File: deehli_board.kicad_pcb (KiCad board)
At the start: 2 copper layers, 84 x 51 mm, 46 parts, among them J1 Servo_Out, J2 PWM_In, J3 Vcc_Out, J4 Conn_01x08_Socket, J5 CAN_Ext, J6 Board_IO, J7 Conn_01x08_Socket, SW1 SW_DPDT_x2, U1 APE1707M-50-HF, U2 LM2576HVT-5, U3 LM2576HVT-5, U4 LM2576HVT-15, U5 LD1117S33TR_SOT223, U6 LM2576HVT-15

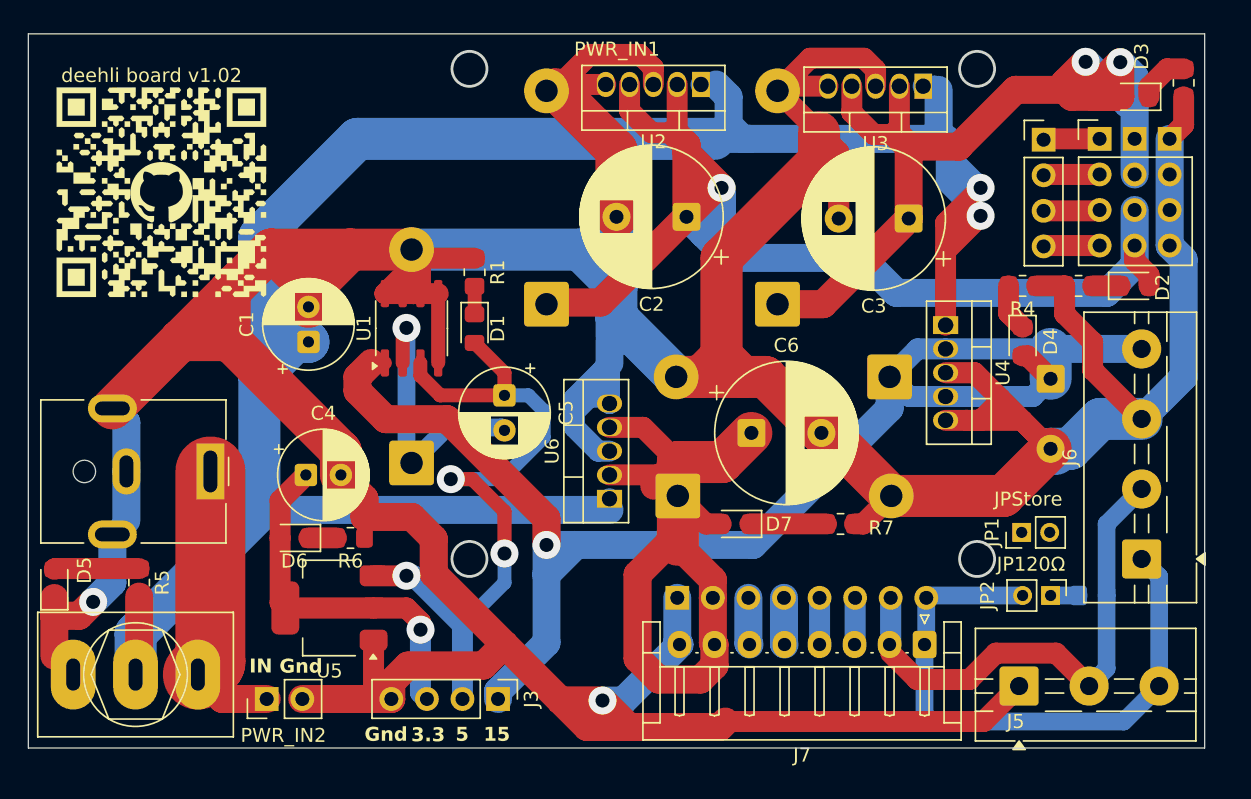
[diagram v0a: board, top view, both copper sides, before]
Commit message: vB-1.01
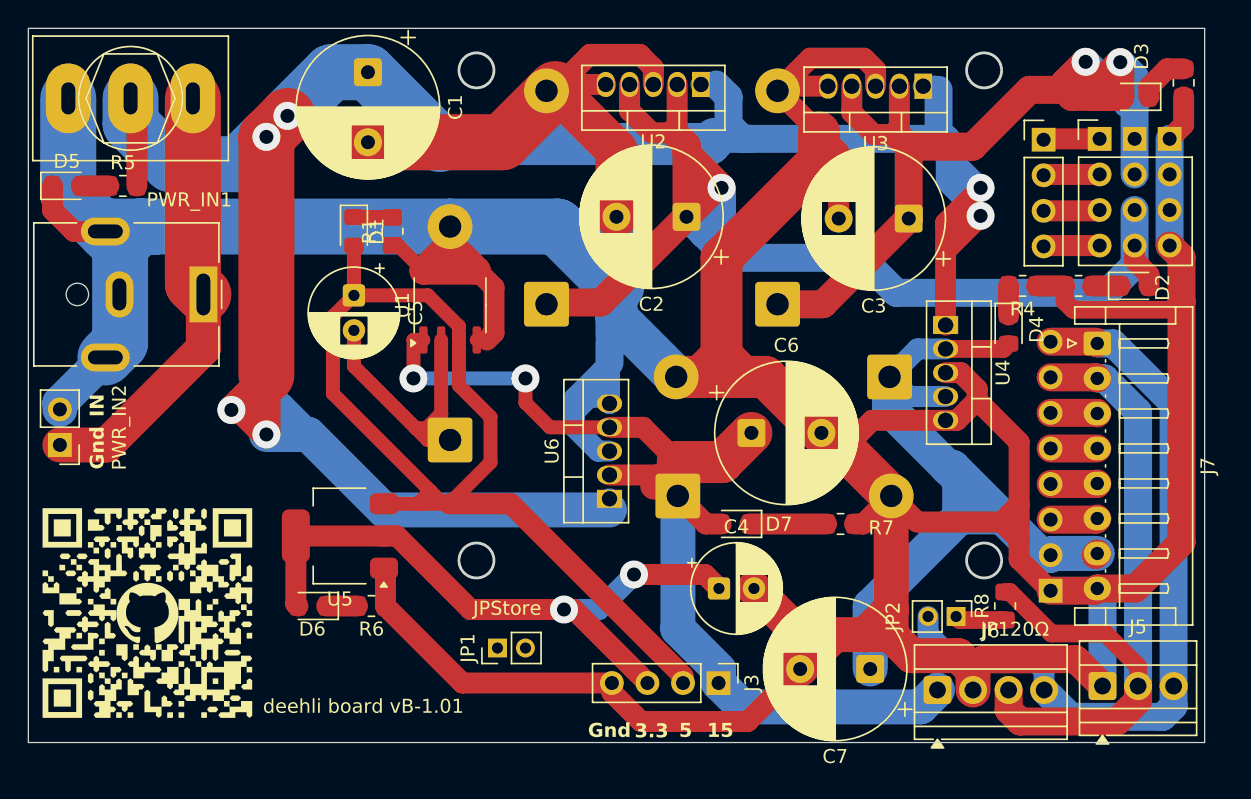
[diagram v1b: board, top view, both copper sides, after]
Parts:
- C1: value Cpol 400uF -> Cpol 1000uF; footprint Capacitor_THT:CP_Radial_D6.3mm_P2.50mm -> Capacitor_THT:CP_Radial_D10.0mm_P5.00mm
- C7, R8: moved to F.Cu
- J4: value Conn_01x08_Socket -> ZDT_Pins
- J5: footprint TerminalBlock:TerminalBlock_MaiXu_MX126-5.0-03P_1x03_P5.00mm -> TerminalBlock:TerminalBlock_Xinya_XY308-2.54-3P_1x03_P2.54mm_Horizontal
- J6: footprint TerminalBlock:TerminalBlock_MaiXu_MX126-5.0-04P_1x04_P5.00mm -> TerminalBlock:TerminalBlock_Xinya_XY308-2.54-4P_1x04_P2.54mm_Horizontal
- J7: value Conn_01x08_Socket -> ZDT_Connector
- moved SW1 41.1 mm to (35.3, 41.0)
- moved JP1 38.3 mm to (61.5, 80.2)
- moved C4 30.6 mm to (77.3, 76.0)
- moved G*** 30.1 mm to (36.5, 77.8)
- moved D5 28.4 mm to (30.8, 47.2), turned to 0 degrees
- moved R5 28.4 mm to (34.8, 47.2), turned to 0 degrees
- moved J4 26.7 mm to (101.0, 76.2), turned to 0 degrees
- moved J7 24.8 mm to (104.3, 58.5), turned to -90 degrees
- moved C7 24.4 mm to (88.1, 81.8), turned to 180 degrees
- moved PWR_IN2 23.4 mm to (30.2, 65.8), turned to 180 degrees
- moved C1 19.7 mm to (52.2, 39.1), turned to -90 degrees
- moved J6 17.3 mm to (92.9, 83.2), turned to 0 degrees
- moved J3 15.8 mm to (77.3, 82.8)
- moved C5 12.9 mm to (51.2, 55.1)
- moved PWR_IN1 12.7 mm to (40.5, 55.0)
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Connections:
- C6 pad 1: 15V_ZDT -> 15V_Other
- C7 pad 1: 15V_Other -> 15V_ZDT
- D11 pad 1: 15V_ZDT -> 15V_Other
- D4 pad 2: 15V_Other -> 15V_ZDT
- D7 pad 2: 15V_ZDT -> 15V_Other
- D8 pad 1: 15V_Other -> 15V_ZDT
- J6 pad 1: CAN_L -> 15V_Other
- J6 pad 2: CAN_H -> GND
- J6 pad 3: GND -> CAN_H
- J6 pad 4: 15V_Other -> CAN_L
- U4 pad 2: 15V_Other -> 15V_ZDT
- U4 pad 4: 15V_Other -> 15V_ZDT
- U6 pad 2: 15V_ZDT -> 15V_Other
- U6 pad 4: 15V_ZDT -> 15V_Other
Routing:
- net 15V_Other: track 104.9 -> 77.6 mm, vias 1 -> 2
- net 5V_Other: track 52.4 -> 73.8 mm, vias 3 -> 0
- net 3.3V_Other: track 26.2 -> 47.0 mm, vias 1 -> 2
- net CAN_H: track 35.7 -> 52.6 mm
- net Net-(SW1A-B): track 161.4 -> 173.7 mm, vias 2 -> 6
- net CAN_L: track 42.9 -> 54.6 mm
- net Net-(PWR_IN2-Pin_1): track 20.5 -> 31.3 mm
- net Net-(D5-A): track 6.08 -> 1.98 mm
- net Net-(JP2-A): track 2.00 -> 3.60 mm
- net Net-(D4-K): track 3.36 -> 2.08 mm
- net 15V_ZDT: track 55.7 -> 56.9 mm
- net GND: track 427.7 -> 428.8 mm, vias 2 -> 0
- net Net-(D12-K): track 20.2 -> 21.3 mm, vias 1 -> 0
- net Net-(D1-K): track 2.00 -> 2.76 mm
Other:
- outline, holes or cut-outs redrawn
- board text added: "deehli board vB-1.01"
- board text removed: "deehli board v1.02"
